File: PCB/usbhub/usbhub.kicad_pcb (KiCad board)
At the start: 2 copper layers, 30.8 x 54.8 mm, 35 parts, among them U1 SL2.1S, U2 SL2.1S

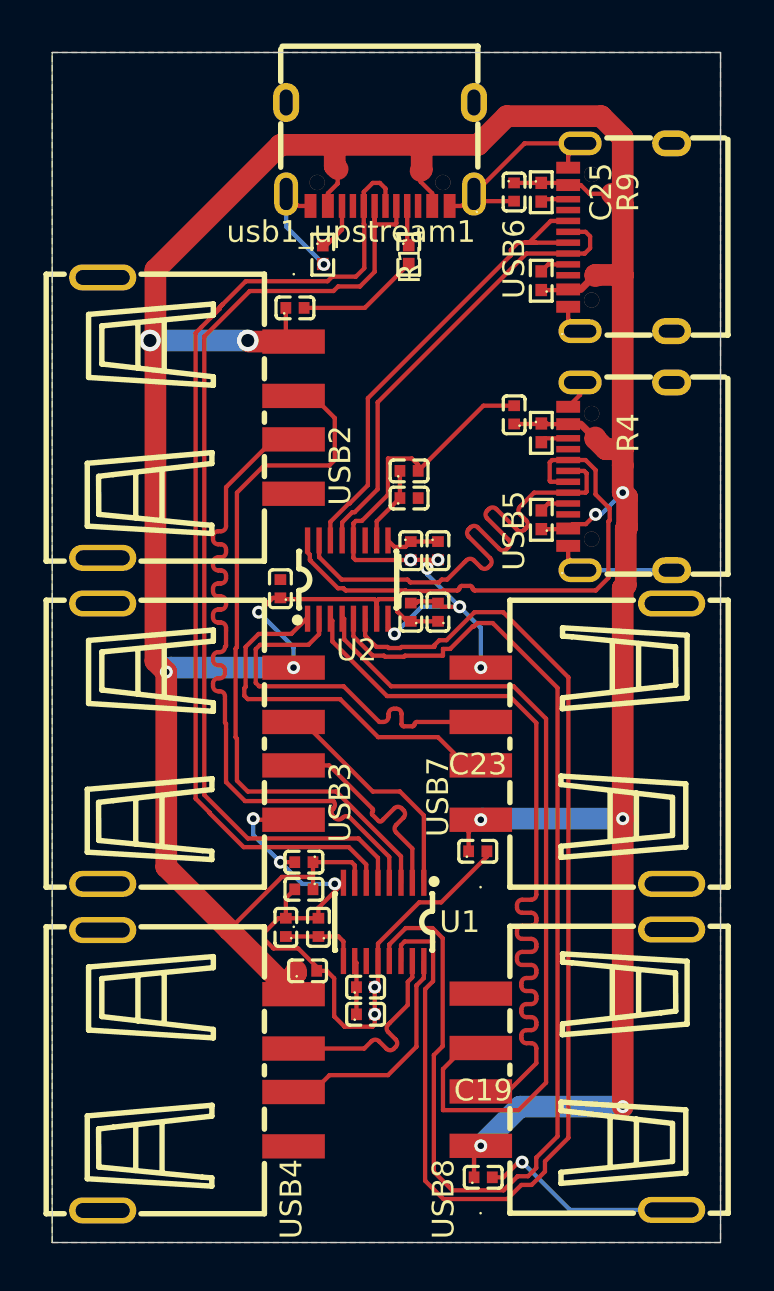
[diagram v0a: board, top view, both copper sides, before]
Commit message: case and assembly
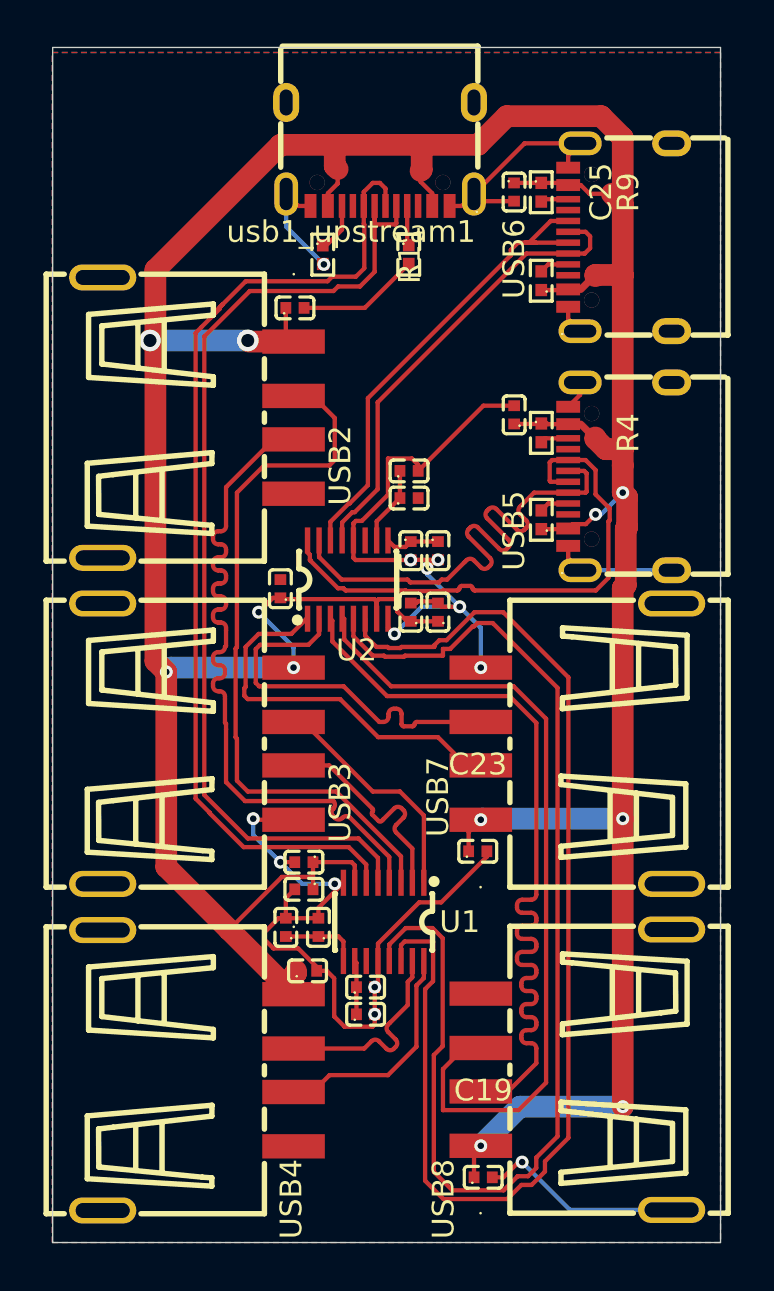
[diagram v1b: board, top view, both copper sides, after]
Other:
- board size 30.8 x 54.8 mm -> 30.7 x 55 mm
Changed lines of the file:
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@@
 	)
 	(gr_rect
-		(start 148.5 41.75)
+		(start 148.524591 41.518764)
 		(end 179.25 96.5)
+		(radius 2)
 		(stroke
 			(width 0.05)
-			(type default)
+			(type solid)
 		)
 		(fill no)
